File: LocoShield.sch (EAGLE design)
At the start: 21 parts, among them J2 RJ12, J3 RJ12, Q1 2N3904, U1 LM393M, U2 LM317LCDR

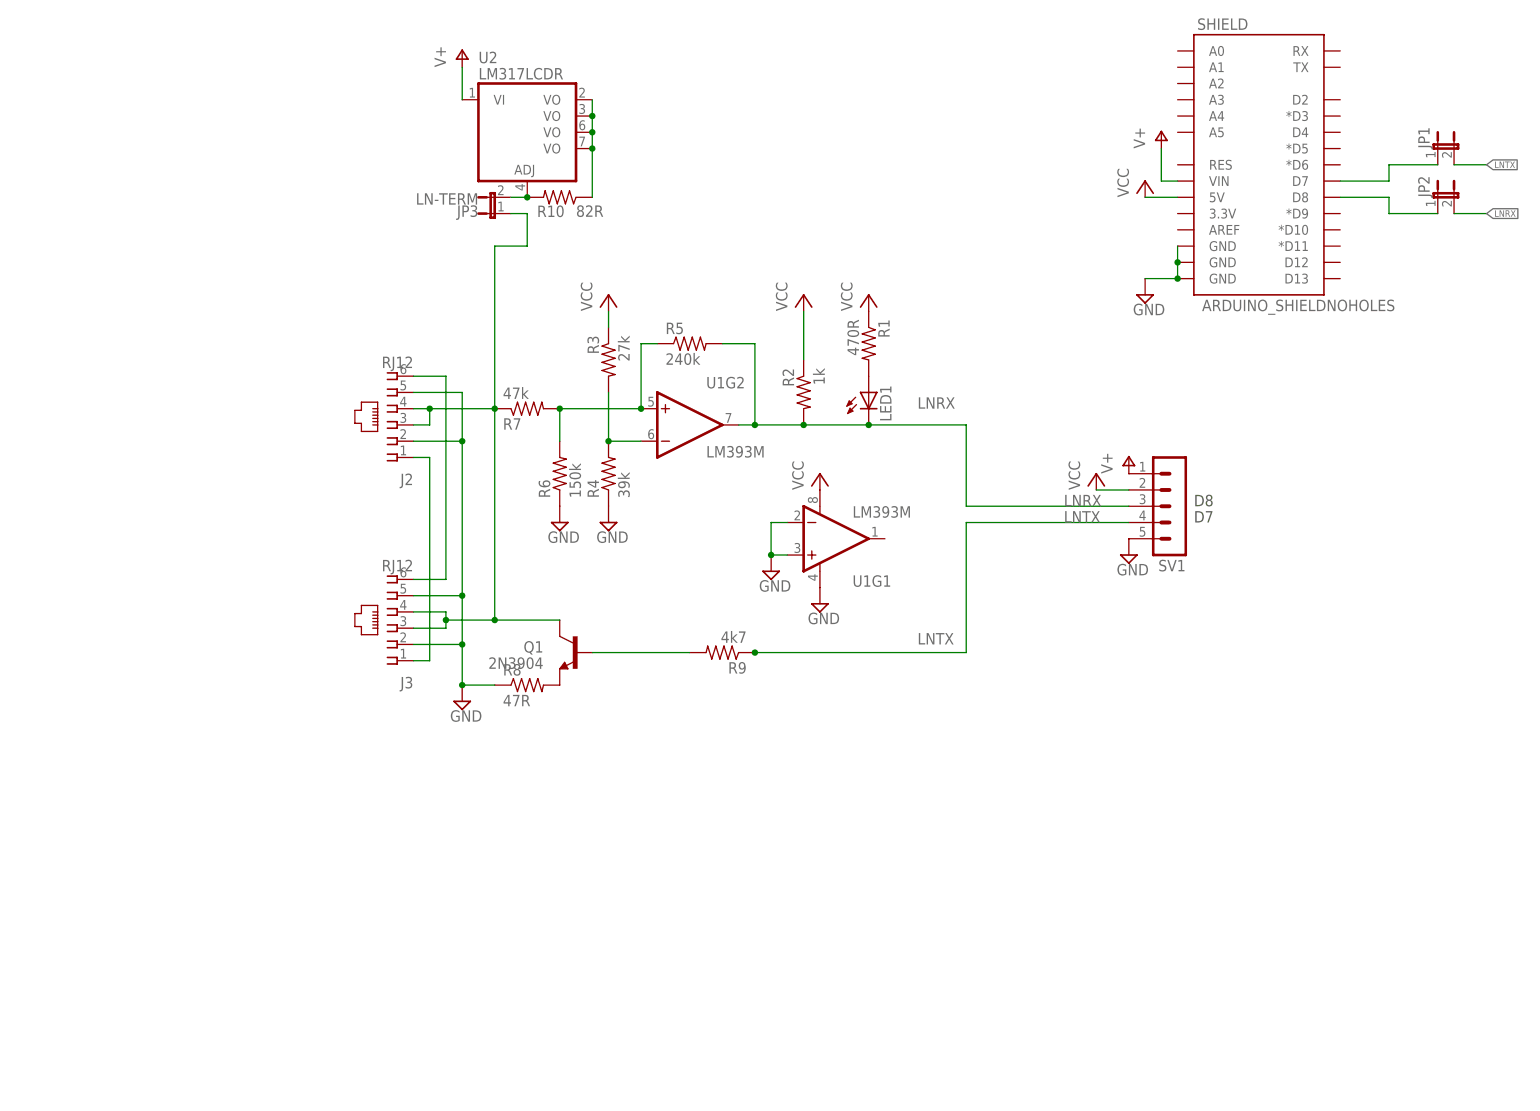
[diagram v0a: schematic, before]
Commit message: 1.4
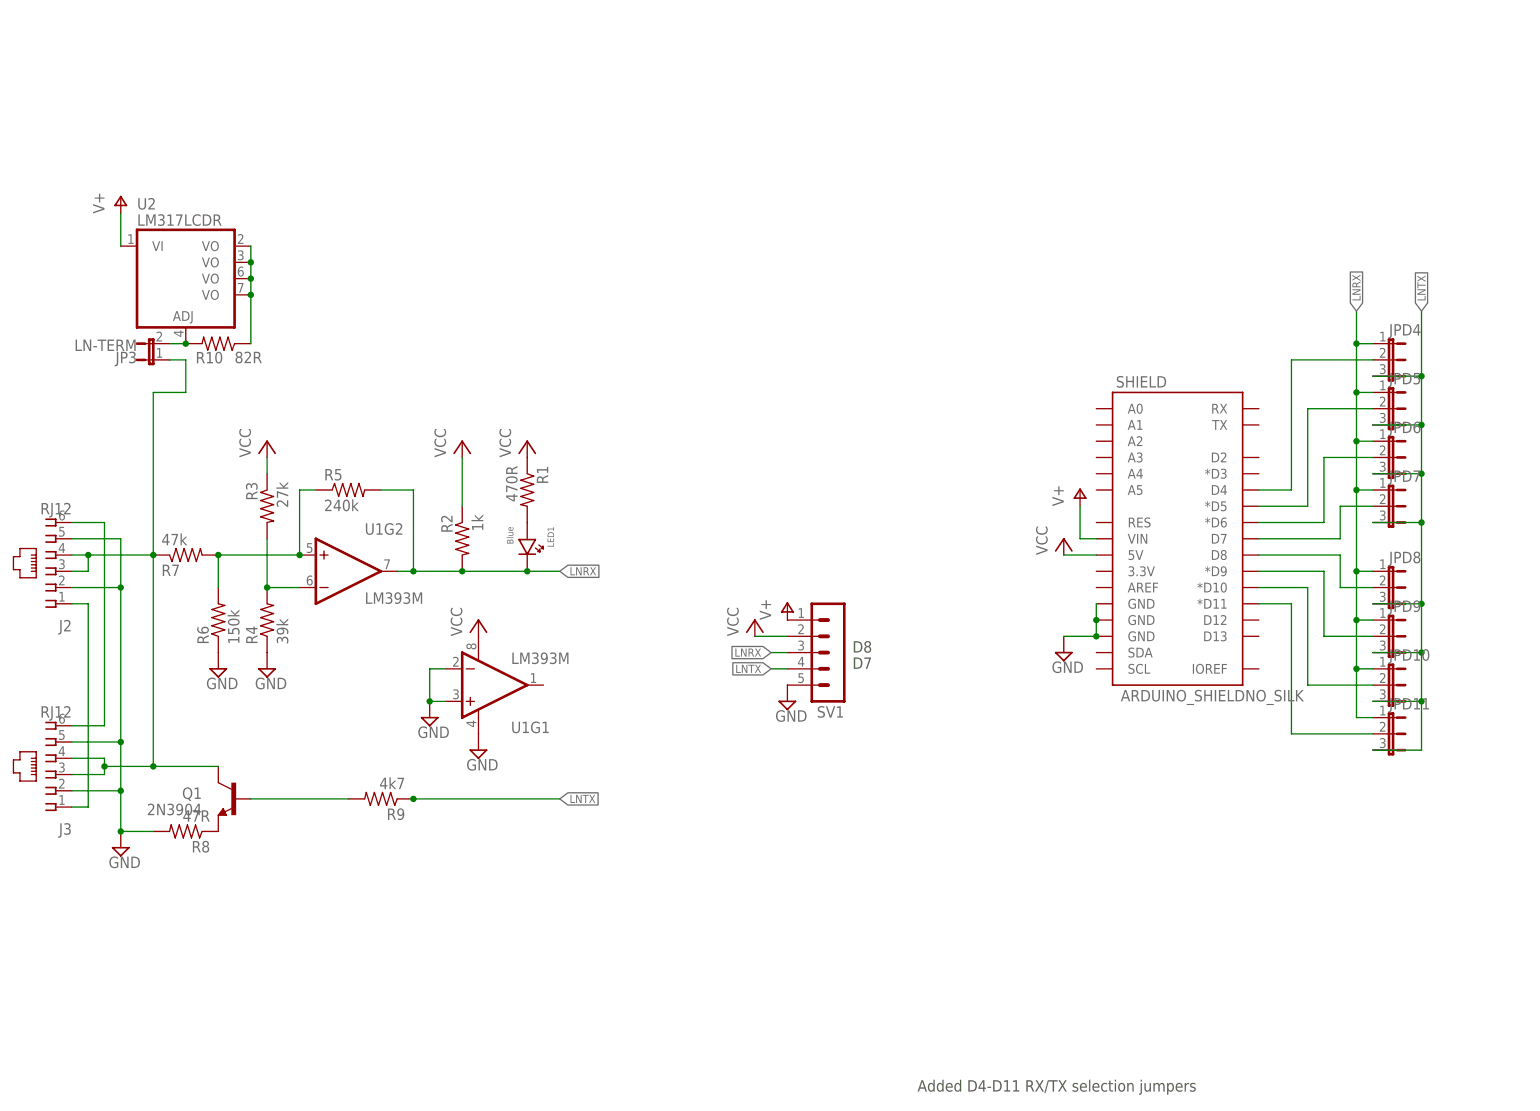
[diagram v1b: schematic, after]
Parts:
- removed JP1, JP2: (no value), MCP:JUMPER-2PTH_LOCK
- added JPD10, JPD11, JPD4, JPD5, JPD6, JPD7, JPD8, JPD9: (no value), MCP:JP2E
- LED1: value (none) -> Blue; device MCP:LEDCHIPLED_0805 -> SPCoast:LED0805-LED
- R1, R2, R3, R4, R5, R6, R7, R8, R9: device rcl:R-US_R0805W -> SPCoast:R0805-RES
- R10: device rcl:R-US_R0805 -> SPCoast:R0805-RES
- SHIELD: value ARDUINO_SHIELDNOHOLES -> ARDUINO_SHIELDNO_SILK; device SparkFun:ARDUINO_SHIELDNOHOLES -> SPCoast:ARDUINO_SHIELDNO_SILK
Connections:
- removed net N$3: JP1.1, SHIELD.D7
- removed net N$4: JP2.1, SHIELD.D8
- new net D10: JPD10.2, SHIELD.*D10
- new net D11: JPD11.2, SHIELD.*D11
- new net D4: JPD4.2, SHIELD.D4
- new net D5: JPD5.2, SHIELD.*D5
- new net D6: JPD6.2, SHIELD.*D6
- new net D7: JPD7.2, SHIELD.D7
- new net D8: JPD8.2, SHIELD.D8
- new net D9: JPD9.2, SHIELD.*D9
- net GND: now also R8.2; no longer R8.1
- net LNRX: now also JPD10.1, JPD11.1, JPD4.1, JPD5.1, JPD6.1, JPD7.1, JPD8.1, JPD9.1; no longer JP2.2
- net LNTX: now also JPD10.3, JPD11.3, JPD4.3, JPD5.3, JPD6.3, JPD7.3, JPD8.3, JPD9.3; no longer JP1.2
- net N$6: now also R8.1; no longer R8.2
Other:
- note added: "1.4"
- note added: "Added D4-D11 RX/TX selection jumpers"
- note removed: "1.3"
- moved on the sheet: J2, J3, JP3, Q1, SV1, U1G1, U1G2, U2
